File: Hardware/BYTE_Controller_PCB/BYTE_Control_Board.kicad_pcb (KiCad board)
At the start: 2 copper layers, 20.8 x 40.6 mm, 11 parts, among them J1 8P8C_Shielded, Q1 2N7002, U1 SeeeduinoXIAO

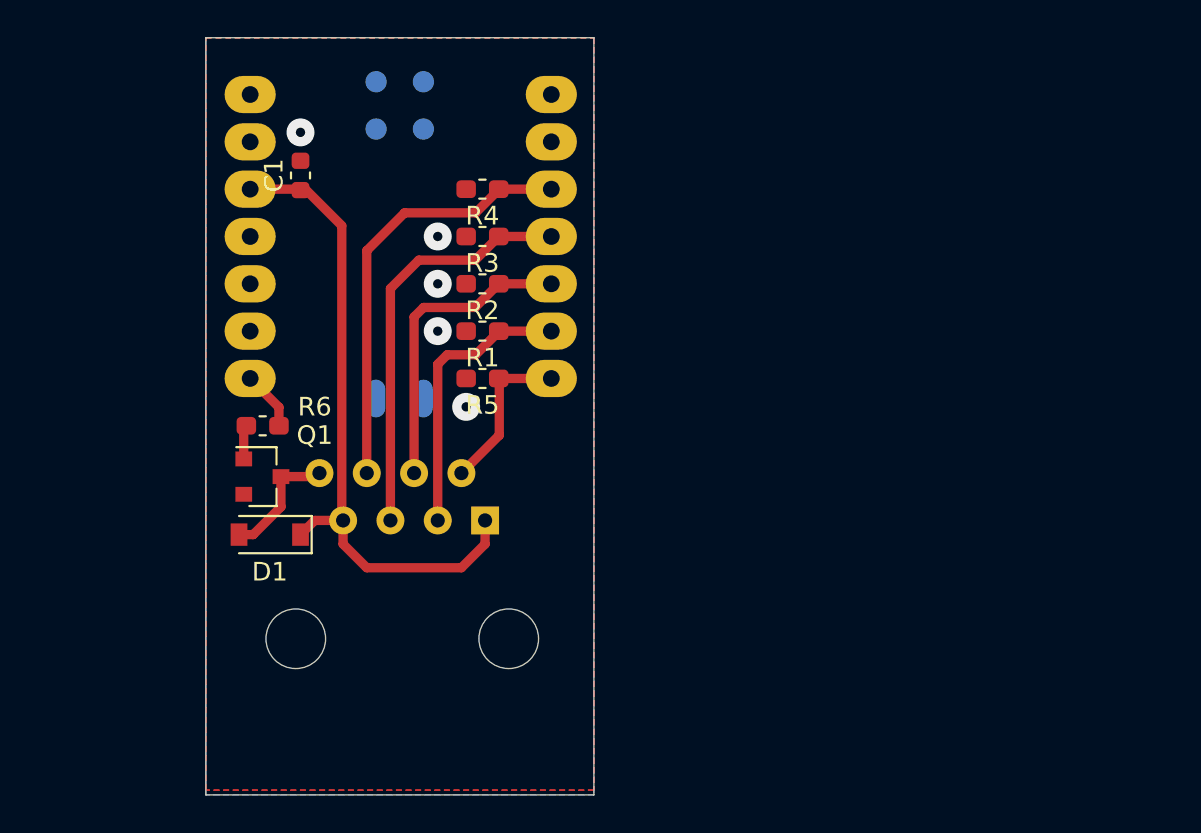
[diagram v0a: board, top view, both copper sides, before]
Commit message: modify controller board
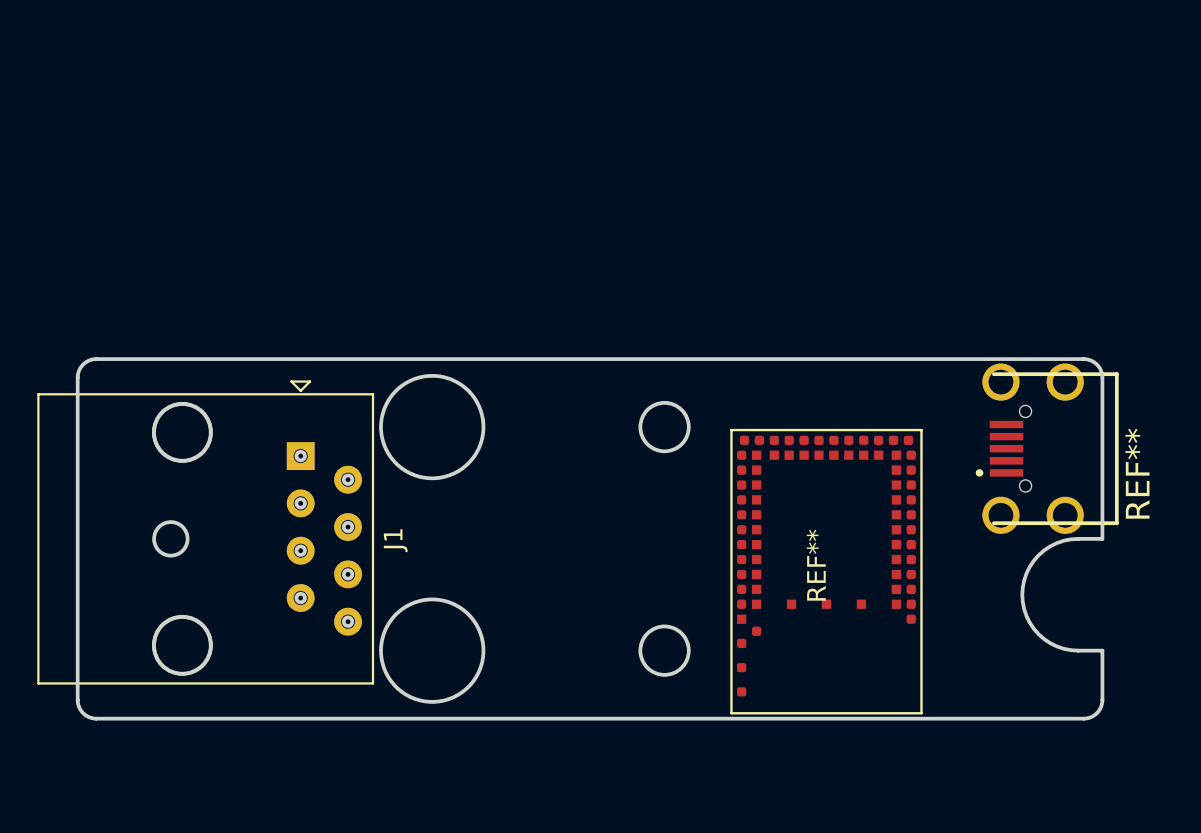
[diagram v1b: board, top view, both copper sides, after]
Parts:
- removed C1: C, Capacitor_SMD:C_0603_1608Metric
- removed D1: D_Schottky, Diode_SMD:D_SOD-123
- removed Q1: 2N7002, Package_TO_SOT_SMD:SOT-23
- removed R1, R2, R3, R4, R5, R6: R_US, Resistor_SMD:R_0603_1608Metric_Pad1.05x0.95mm_HandSolder
- removed U1: SeeeduinoXIAO, XIAO:XIAO-MOUDLE14P-2.54-21X17.8MM_Through_Hole
- added REF**: U254051N4BH806, Connectors:U254051N4BH806, F.Cu at (172.2, 105.4)
- added REF**: BL653, Controller:BL653_v5, F.Cu at (160.3, 111.7)
- J1: moved to F.Cu
- moved J1 10.5 mm to (132.1, 105.8), turned to 270 degrees
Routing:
- net Net-(C1-Pad1): track 35.4 -> 0.00 mm
- net Net-(J1-Pad6): track 23.2 -> 0.00 mm
- net Net-(J1-Pad5): track 22.2 -> 0.00 mm
- net Net-(J1-Pad4): track 16.5 -> 0.00 mm
- net Net-(J1-Pad3): track 15.2 -> 0.00 mm
- net Net-(J1-Pad2): track 8.76 -> 0.00 mm
- net Net-(D1-Pad2): track 6.73 -> 0.00 mm
- net Net-(R6-Pad1): track 3.18 -> 0.00 mm
- net Net-(Q1-Pad1): track 1.84 -> 0.00 mm
- net GND: vias 5 -> 0
- removed copper zone on F.Cu, net (none)
- removed copper zone on B.Cu, net GND
- removed copper zone on F.Cu, net GND
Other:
- board size 20.8 x 40.6 mm -> 55 x 19.3 mm
